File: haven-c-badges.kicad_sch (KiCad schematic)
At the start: 5 parts, among them U1 NT3H2111W0FHKH

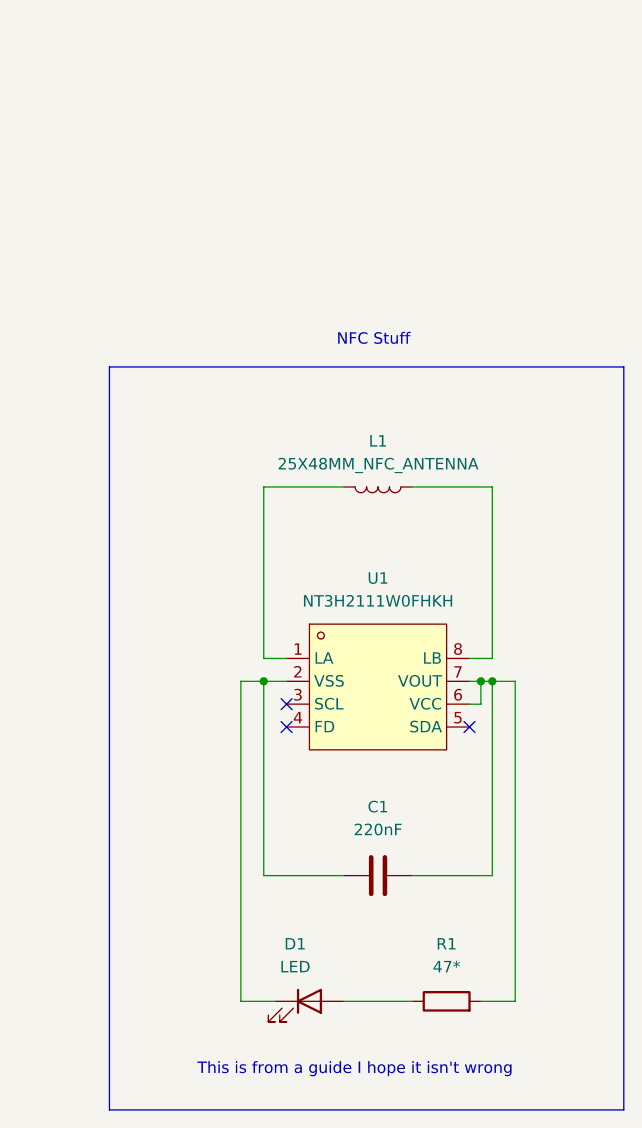
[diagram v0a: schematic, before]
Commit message: idk some scaling adjustment things
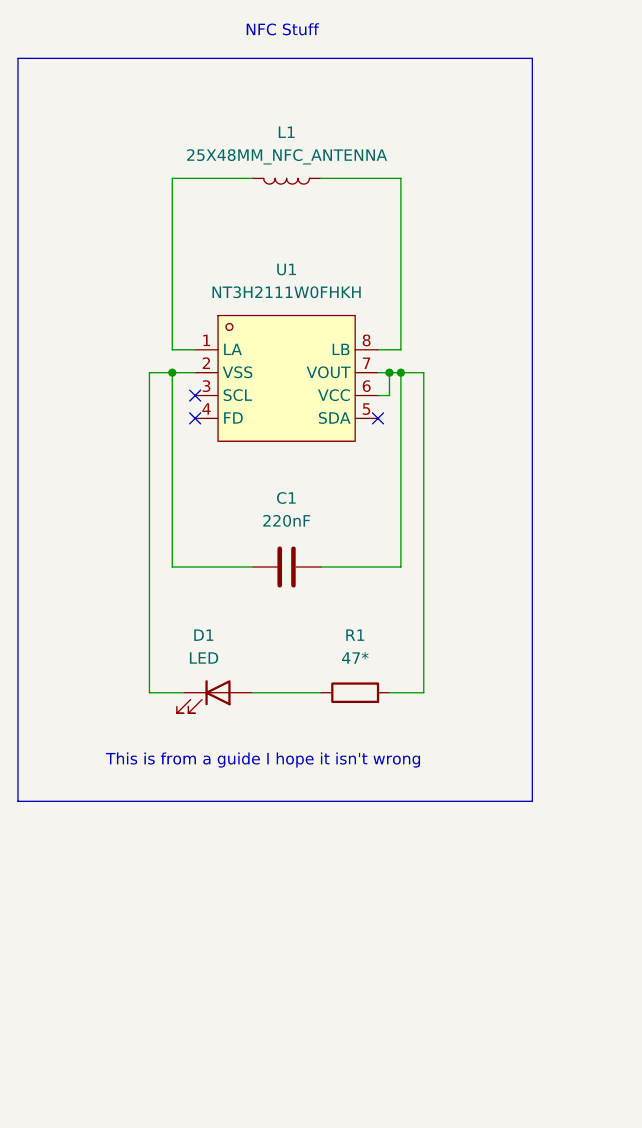
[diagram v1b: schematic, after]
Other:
- moved on the sheet: C1, D1, L1, R1, U1
